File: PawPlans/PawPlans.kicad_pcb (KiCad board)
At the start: 2 copper layers, 80 x 66 mm, 7 parts

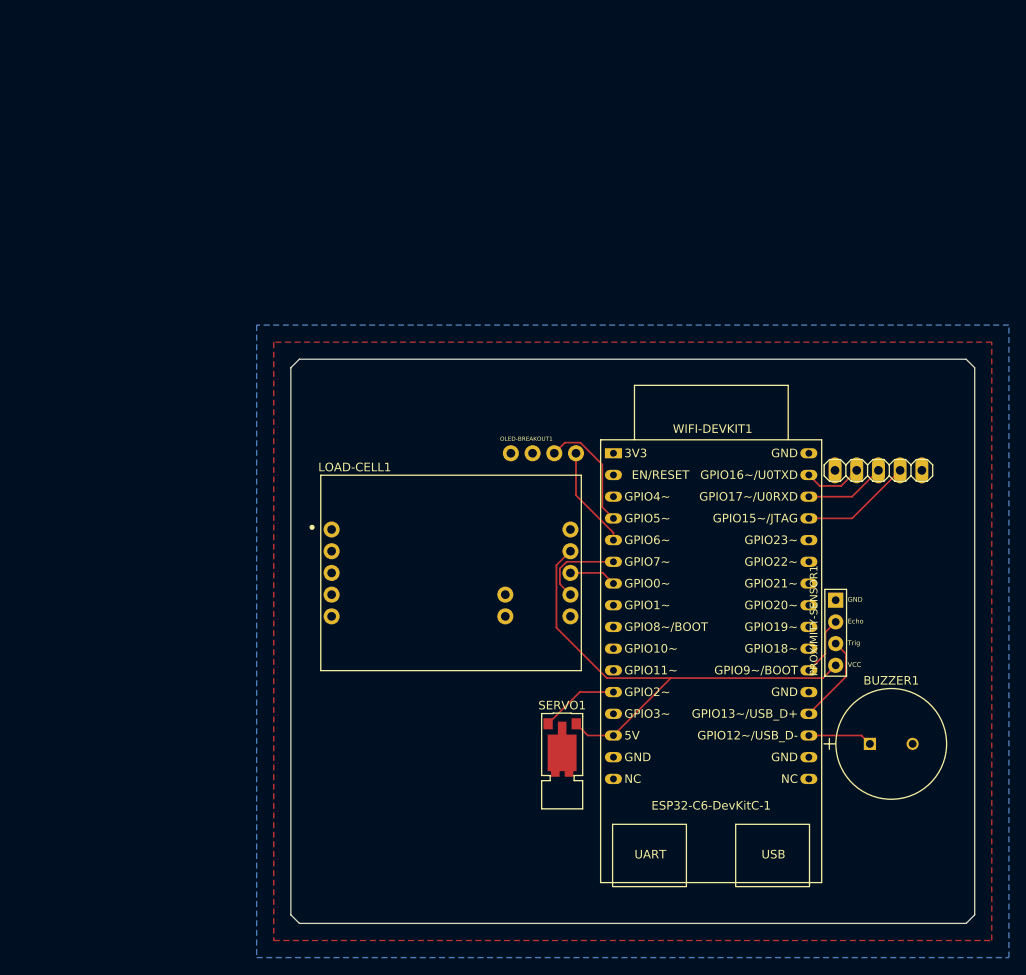
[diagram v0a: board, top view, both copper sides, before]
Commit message: Completely revamped the schematic and PCB, cleaned up project files
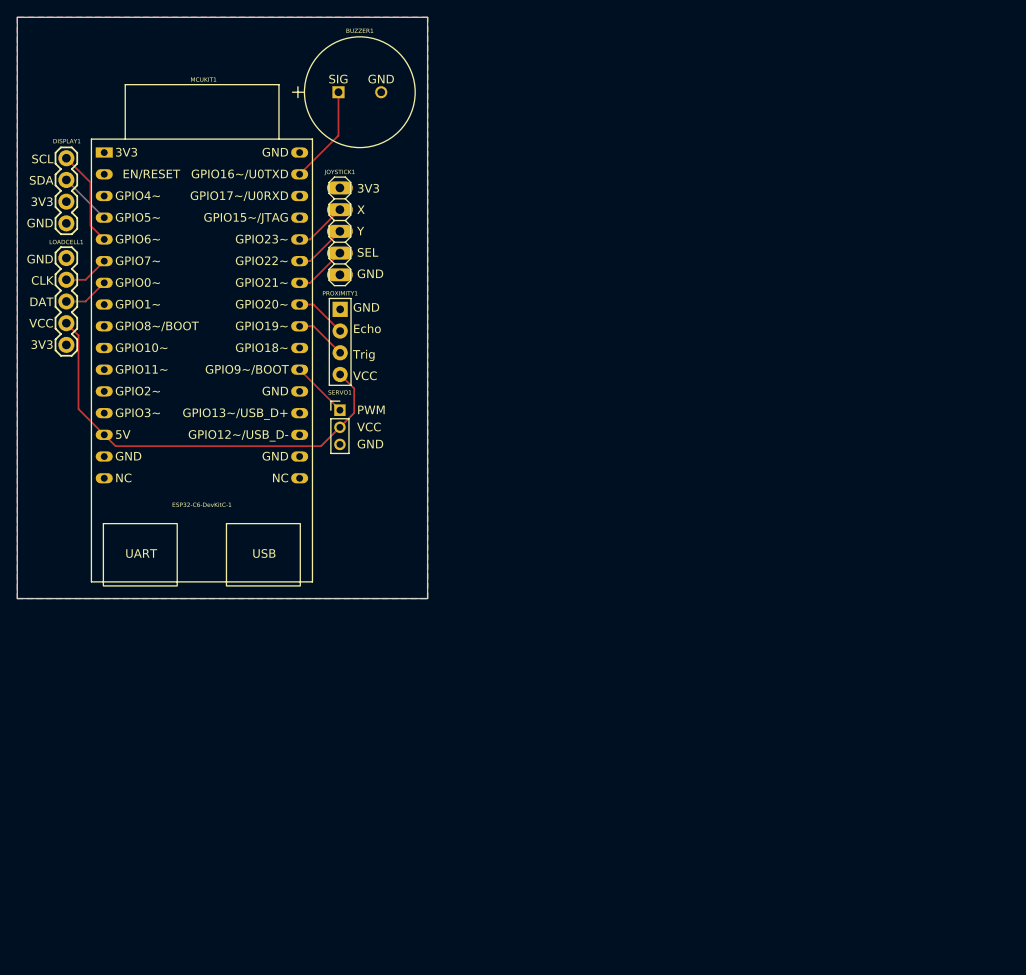
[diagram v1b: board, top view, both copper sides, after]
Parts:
- removed LOAD-CELL1: SEN-13879, Parts:SPARKFUN_SEN-13879
- removed PROXIMITY-SENSOR1: ~, Ultrasonic Sensor HC-SR04:HC-SR04_FOOTPRINT
- added LOADCELL1: ~, SparkFun_HX711_Load_Cell_Amplifier_SEN-13879:SPARKFUN-CONNECTORS_1X05, F.Cu at (83.7, 66.3)
- added PROXIMITY1: ~, Ultrasonic_Proximity_Sensor_HC-SR04:HC-SR04_FOOTPRINT, F.Cu at (115.8, 66.0)
- BUZZER1: footprint Parts:XTAL_PS1240P02BT_TDK -> TDK_Piezo_Buzzer_PS1240P02BT:XTAL_PS1240P02BT_TDK
- DISPLAY1: renamed from OLED-BREAKOUT1; footprint Qwiic_OLED_1.3in:SPARKX_1X04_NO_SILK -> SparkFun_Qwiic_OLED_128x64_LCD-23453:SPARKX_1X04
- JOYSTICK1: footprint Parts:1X05 -> Adafruit_Joystick_512:PINHEAD_1X05
- MCUKIT1: renamed from WIFI-DEVKIT1; footprint Espressif:ESP32-C6-DevKitC-1 -> Espressif_ESP32:ESP32-C6-DevKitC-1
- SERVO1: footprint Motors:Vybronics_VZ30C1T8219732L -> Connector_PinHeader_2.00mm:PinHeader_1x03_P2.00mm_Vertical
- moved BUZZER1 98.4 mm to (115.6, 36.8)
- moved MCUKIT1 69.2 mm to (88.2, 43.8)
- moved JOYSTICK1 68.9 mm to (115.7, 53.0), turned to -90 degrees
- moved DISPLAY1 58.5 mm to (83.7, 52.1), turned to 90 degrees
- moved SERVO1 48.6 mm to (115.7, 74.0)
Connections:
- net Net-(OLED-BREAKOUT1-SCL) renamed /DSPSCL
- net Net-(OLED-BREAKOUT1-SDA) renamed /DSPSDA
- BUZZER1 pad 1: Net-(WIFI-DEVKIT1-GPIO12/USB_D-) -> /PZOSIG
- JOYSTICK1 pad 2: Net-(WIFI-DEVKIT1-GPIO16/U0TXD) -> /JOYX
- JOYSTICK1 pad 3: Net-(WIFI-DEVKIT1-GPIO17/U0RXD) -> /JOYY
- JOYSTICK1 pad 4: Net-(WIFI-DEVKIT1-GPIO15/JTAG) -> /JOYSEL
- MCUKIT1 pad 12: Net-(SERVO1-PWM) -> unconnected-(MCUKIT1-GPIO2-Pad12)
- MCUKIT1 pad 19: Net-(WIFI-DEVKIT1-GPIO12/USB_D-) -> unconnected-(MCUKIT1-GPIO12/USB_D--Pad19)
- MCUKIT1 pad 20: Net-(WIFI-DEVKIT1-GPIO13/USB_D+) -> unconnected-(MCUKIT1-GPIO13/USB_D+-Pad20)
- MCUKIT1 pad 22: Net-(WIFI-DEVKIT1-GPIO9/BOOT) -> /SRVPWM
- MCUKIT1 pad 24: unconnected-(WIFI-DEVKIT1-GPIO19-Pad24) -> /PRXTRG
- MCUKIT1 pad 25: unconnected-(WIFI-DEVKIT1-GPIO20-Pad25) -> /PRXECH
- MCUKIT1 pad 26: unconnected-(WIFI-DEVKIT1-GPIO21-Pad26) -> /JOYSEL
- MCUKIT1 pad 27: unconnected-(WIFI-DEVKIT1-GPIO22-Pad27) -> /JOYY
- MCUKIT1 pad 28: unconnected-(WIFI-DEVKIT1-GPIO23-Pad28) -> /JOYX
- MCUKIT1 pad 29: Net-(WIFI-DEVKIT1-GPIO15/JTAG) -> unconnected-(MCUKIT1-GPIO15/JTAG-Pad29)
- MCUKIT1 pad 30: Net-(WIFI-DEVKIT1-GPIO17/U0RXD) -> unconnected-(MCUKIT1-GPIO17/U0RXD-Pad30)
- MCUKIT1 pad 31: Net-(WIFI-DEVKIT1-GPIO16/U0TXD) -> /PZOSIG
- MCUKIT1 pad 6: Net-(LOAD-CELL1-CLK) -> /LDCCLK
- MCUKIT1 pad 7: Net-(LOAD-CELL1-DAT) -> /LDCDAT
- SERVO1 pad 1: Net-(SERVO1-PWM) -> /SRVPWM
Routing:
- net Net-(WIFI-DEVKIT1-GPIO15/JTAG): track 13.0 -> 0.00 mm
- net /PZOSIG: track 0.00 -> 11.5 mm
- net Net-(WIFI-DEVKIT1-GPIO13/USB_D+): track 10.5 -> 0.00 mm
- net Net-(LOAD-CELL1-CLK): track 10.2 -> 0.00 mm
- net Net-(WIFI-DEVKIT1-GPIO17/U0RXD): track 9.42 -> 0.00 mm
- net Net-(SERVO1-PWM): track 9.19 -> 0.00 mm
- net /VCC: track 59.8 -> 51.5 mm
- net /DSPSDA: track 14.0 -> 6.26 mm
- net Net-(WIFI-DEVKIT1-GPIO12/USB_D-): track 7.55 -> 0.00 mm
- net Net-(WIFI-DEVKIT1-GPIO9/BOOT): track 6.97 -> 0.00 mm
- net Net-(WIFI-DEVKIT1-GPIO16/U0TXD): track 6.89 -> 0.00 mm
- net /SRVPWM: track 0.00 -> 6.69 mm
- net /JOYX: track 0.00 -> 6.15 mm
- net /JOYY: track 0.00 -> 6.15 mm
- net /JOYSEL: track 0.00 -> 6.15 mm
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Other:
- board size 80 x 66 mm -> 48 x 68 mm
